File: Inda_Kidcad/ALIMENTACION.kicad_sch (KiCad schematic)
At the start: 15 parts, among them U6 CN3903, U7 AMS1117-5.0

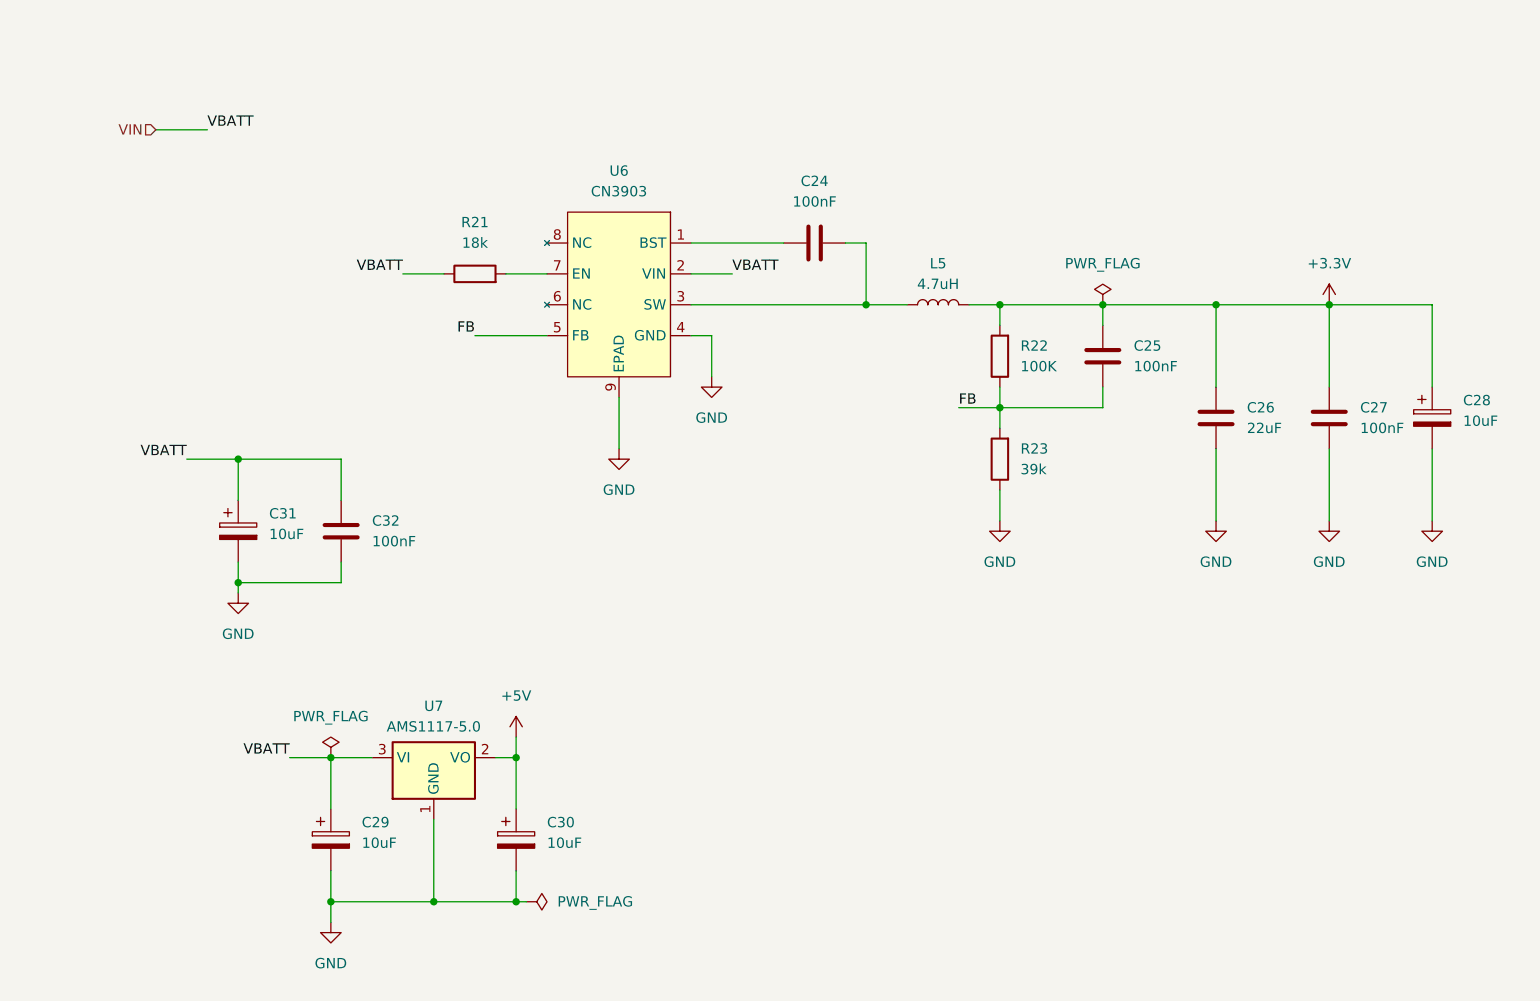
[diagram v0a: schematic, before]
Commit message: Version 2 De Sumo Inda
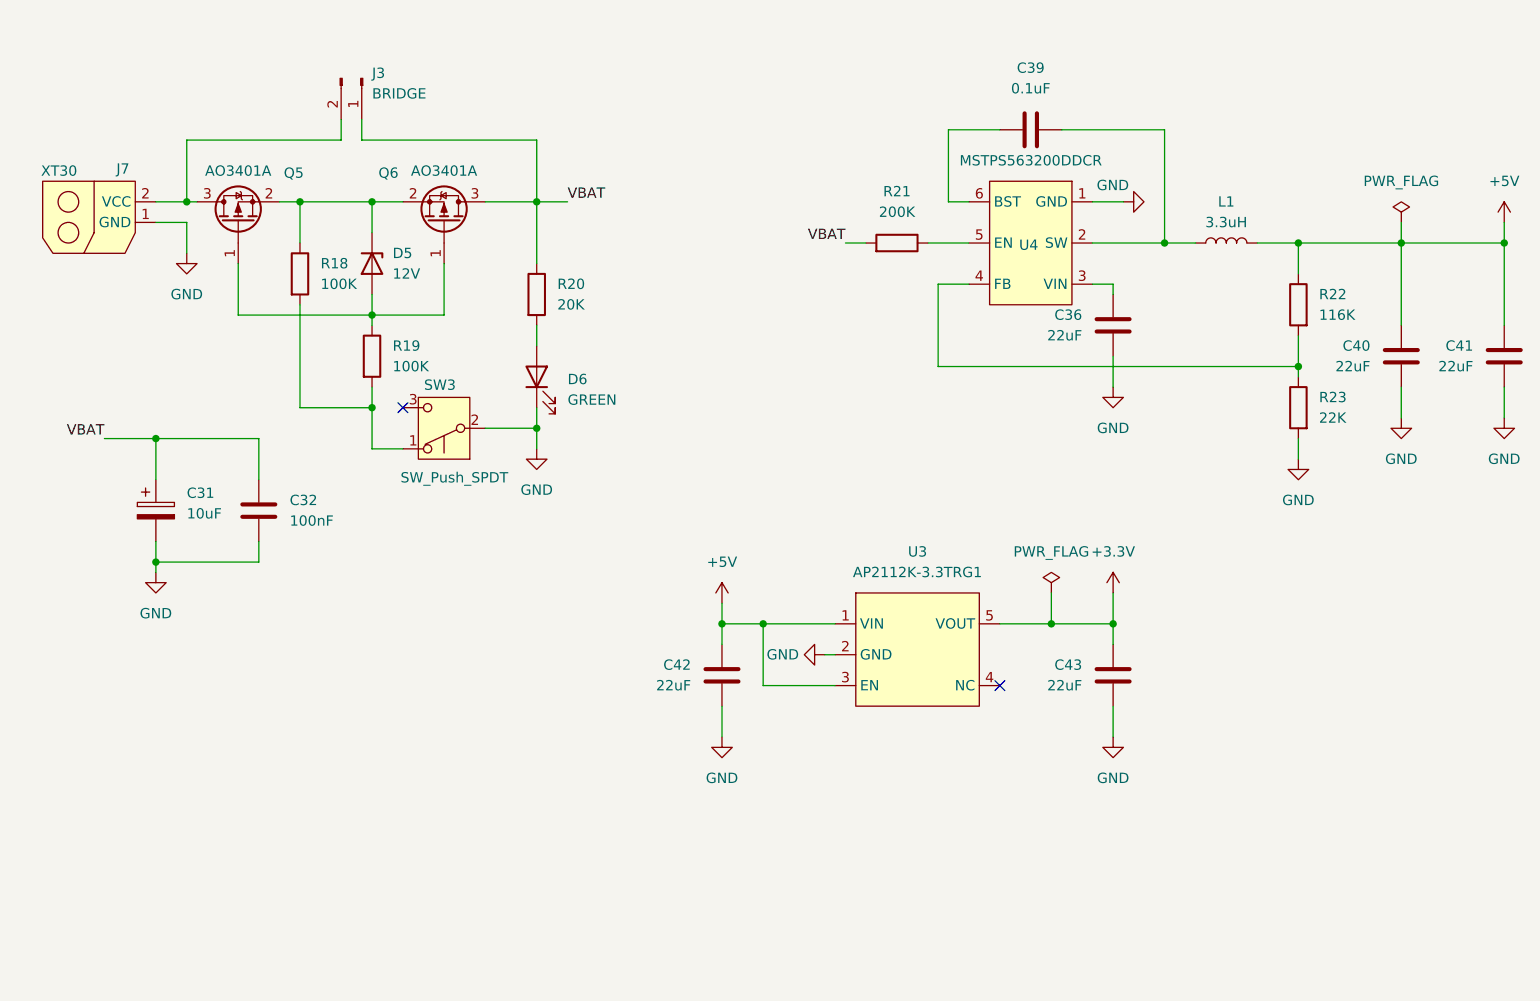
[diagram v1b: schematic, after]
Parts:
- removed C24, C25, C27: 100nF, Capacitor_SMD:C_0603_1608Metric, symbol Device:C
- removed C26: 22uF, Capacitor_SMD:C_0603_1608Metric, symbol Device:C
- removed C28: 10uF, Capacitor_SMD:CP_Elec_4x5.8, symbol Device:C_Polarized
- removed C29, C30: 10uF, Capacitor_SMD:C_1206_3216Metric_Pad1.33x1.80mm_HandSolder, symbol Device:C_Polarized
- removed L5: 4.7uH, Inductor_SMD:L_Wuerth_HCM-7050, symbol Device:L
- removed U6: CN3903, Package_SO:HSOP-8-1EP_3.9x4.9mm_P1.27mm_EP2.41x3.1mm, symbol Micromouse_Library:CN3903
- removed U7: AMS1117-5.0, Package_TO_SOT_SMD:SOT-223-3_TabPin2, symbol Regulator_Linear:AMS1117-5.0
- added C36, C40, C41, C42, C43: 22uF, Capacitor_SMD:C_0603_1608Metric, symbol Device:C
- added C39: 0.1uF, Capacitor_SMD:C_0603_1608Metric, symbol Device:C
- added D5: 12V, Resistor_SMD:R_1206_3216Metric_Pad1.30x1.75mm_HandSolder, symbol Device:D_Zener
- added D6: GREEN, LED_SMD:LED_1206_3216Metric_Pad1.42x1.75mm_HandSolder, symbol Device:LED
- added J3: BRIDGE, Connector_PinHeader_2.54mm:PinHeader_1x02_P2.54mm_Vertical, symbol Connector:Conn_01x02_Pin
- added J7: XT30, Connector_AMASS:AMASS_XT30U-F_1x02_P5.0mm_Vertical, symbol LIB_CONECTORES:Conector_XT30
- added L1: 3.3uH, symbol Device:L
- added Q5, Q6: AO3401A, Package_TO_SOT_SMD:SOT-23, symbol Transistor_FET:AO3401A
- added R18, R19: 100K, Resistor_SMD:R_0805_2012Metric_Pad1.20x1.40mm_HandSolder, symbol Device:R
- added R20: 20K, Resistor_SMD:R_0805_2012Metric_Pad1.20x1.40mm_HandSolder, symbol Device:R
- added SW3: SW_Push_SPDT, Button_Switch_SMD:SW_SPDT_PCM12, symbol Switch:SW_Push_SPDT
- added U3: AP2112K-3.3TRG1, Package_TO_SOT_SMD:SOT-23-5, symbol LIB_REGULADORES:AP2112K-3.3TRG1
- added U4: MSTPS563200DDCR, Package_TO_SOT_SMD:SOT-23-6, symbol LIB_REGULADORES:MSTPS563200DDCR_BUCK
- R21: value 18k -> 200K; footprint Resistor_SMD:R_0805_2012Metric_Pad1.20x1.40mm_HandSolder -> Resistor_SMD:R_0603_1608Metric_Pad0.98x0.95mm_HandSolder
- R22: value 100K -> 116K; footprint Resistor_SMD:R_0805_2012Metric_Pad1.20x1.40mm_HandSolder -> Resistor_SMD:R_0603_1608Metric_Pad0.98x0.95mm_HandSolder
- R23: value 39k -> 22K; footprint Resistor_SMD:R_0805_2012Metric_Pad1.20x1.40mm_HandSolder -> Resistor_SMD:R_0603_1608Metric_Pad0.98x0.95mm_HandSolder
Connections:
- net +3.3V: now also C43.2, U3.5 (VOUT); no longer R22.2
- net +5V: now also R22.1, C40.2, C41.2, C42.2, L1.1, U3.1 (VIN), U3.3 (EN)
- net GND: now also R23.2, C36.1, C40.1, C41.1, C42.1, C43.1, D6.1 (K), J7.1 (GND), SW3.2 (B), U3.2 (GND), U4.1 (GND); no longer R23.1
- net VBAT: now reaches R21.2
- net VBAT: now also C31.1, C32.2, J3.1 (Pin_1), Q6.3 (D), R20.1
- removed net FB: R22.1, R23.2
- removed net VIN: C31.1, C32.2, R21.1
- new net: J3.2 (Pin_2), J7.2 (VCC), Q5.3 (D)
- new net: D5.2 (A), Q5.1 (G), Q6.1 (G), R19.1
- new net: D5.1 (K), Q5.2 (S), Q6.2 (S), R18.1
- new net: D6.2 (A), R20.2
- new net: R18.2, R19.2, SW3.1 (A)
- new net: R22.2, R23.1, U4.4 (FB)
- new net: C39.1, U4.6 (BST)
- new net: C39.2, L1.2, U4.2 (SW)
- new net: R21.1, U4.5 (EN)
- new net: C36.2, U4.3 (VIN)
- no-connect marks 0 -> 2
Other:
- moved on the sheet: C31, C32

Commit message: Se cambia simbolos como huellas, se coloca solo mosfet para interruptor y se empieza con pcb
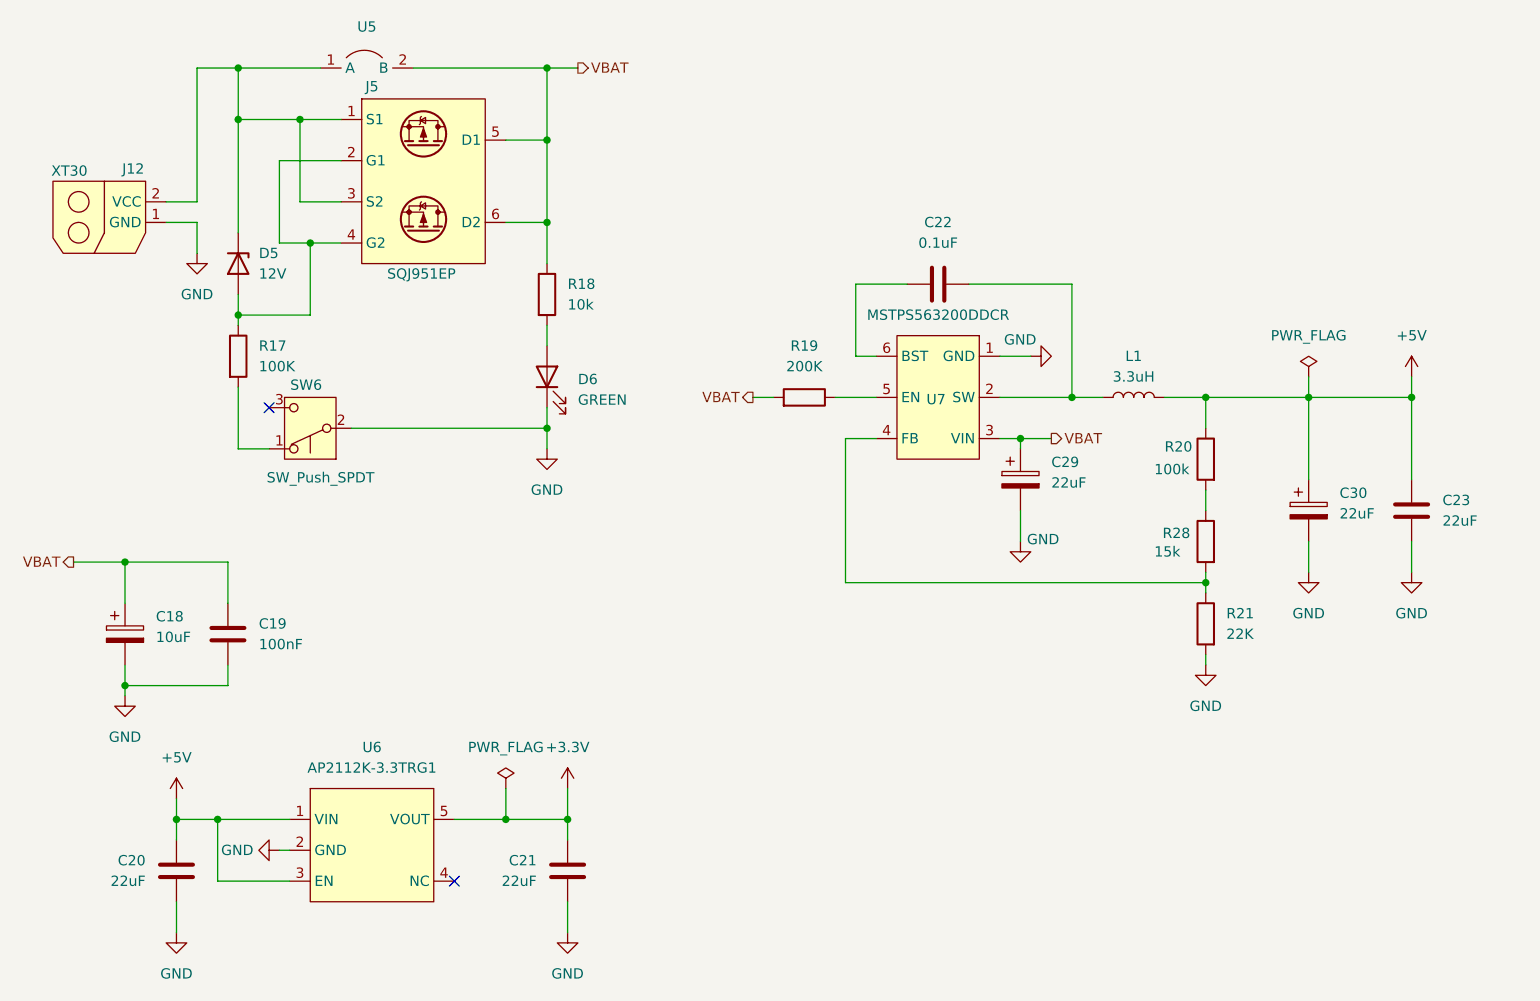
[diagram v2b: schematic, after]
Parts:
- removed C36, C40, C41: 22uF, Capacitor_SMD:C_0603_1608Metric, symbol Device:C
- removed J3: BRIDGE, Connector_PinHeader_2.54mm:PinHeader_1x02_P2.54mm_Vertical, symbol Connector:Conn_01x02_Pin
- removed Q5, Q6: AO3401A, Package_TO_SOT_SMD:SOT-23, symbol Transistor_FET:AO3401A
- removed R18: 100K, Resistor_SMD:R_0805_2012Metric_Pad1.20x1.40mm_HandSolder, symbol Device:R
- added C23: 22uF, Capacitor_SMD:C_0603_1608Metric, symbol Device:C
- added C29, C30: 22uF, Capacitor_Tantalum_SMD:CP_EIA-3528-15_AVX-H_HandSolder, symbol Device:C_Polarized
- added J5: SQJ951EP, Package_SO:PowerPAK_SO-8_Dual, symbol LIB_MOSFET_BJT:SQJ951EP-T1_BE3
- added R28: 15k, Resistor_SMD:R_0603_1608Metric_Pad0.98x0.95mm_HandSolder, symbol Device:R
- added U5: (no value), Footprint:BRIDGE_2P, symbol LIB_CONECTORES:BRIDGE_2P
- J12: renamed from J7; footprint Connector_AMASS:AMASS_XT30U-F_1x02_P5.0mm_Vertical -> Footprint:XT30_H_M
- L1: footprint (none) -> Inductor_SMD:L_Sunlord_MWSA0402S
- R18: renamed from R20; value 20K -> 10k
- R20: renamed from R22; value 116K -> 100k
- renumbered C31 to C18, C32 to C19, C42 to C20, C43 to C21, C39 to C22, R19 to R17, R21 to R19, R23 to R21, SW3 to SW6, U3 to U6, U4 to U7
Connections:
- net +5V: now also C23.2, C30.1
- net GND: now also C23.1, C29.2, C30.2
- net VBAT: now also U7.3 (VIN), C29.1, J5.5 (D1), J5.6 (D2), U5.2 (B)
- net at J12.2 (VCC): now also D5.1 (K), J5.1 (S1), J5.3 (S2), U5.1 (A)
- net at D5.2 (A), R17.1: now also J5.2 (G1), J5.4 (G2)
- net at R21.1, U7.4 (FB): now also R28.2; no longer R20.2
- new net: R20.2, R28.1
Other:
- moved on the sheet: C18, C19, C20, C21, C22, D5, D6, J12, L1, R17, R18, R19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
